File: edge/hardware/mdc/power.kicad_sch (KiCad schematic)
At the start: 1 part, among them J2 Screw_Terminal_01x02

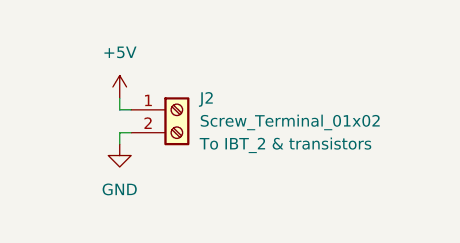
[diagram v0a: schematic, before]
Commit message: rev3.0 schematics
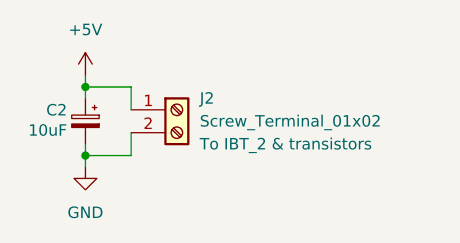
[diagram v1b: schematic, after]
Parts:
- added C2: 10uF, symbol Device:C_Polarized_Small
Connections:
- net +5V: now also C2.1
- net GND: now also C2.2
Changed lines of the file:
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@@
 	(title_block
 		(title "Power")
-		(date "2026-08-08")
+		(date "2026-08-09")
 		(rev "3.0")
 		(comment 1 "Department of EECS- AIoT and Energy Management Lab")
@@
 		(comment 4 "Student: Purit Hongjirakul 黃子奇")
 	)
-	(wire
-		(pts
-			(xy 135.89 100.33) (xy 135.89 99.06)
-		)
-		(stroke
-			(width 0)
-			(type default)
-		)
-	)
-	(wire
-		(pts
-			(xy 135.89 102.87) (xy 137.16 102.87)
-		)
-		(stroke
-			(width 0)
-			(type default)
-		)
-	)
-	(wire
-		(pts
-			(xy 135.89 104.14) (xy 135.89 102.87)
-		)
-		(stroke
-			(width 0)
-			(type default)
-		)
-	)
-	(wire
-		(pts
-			(xy 137.16 100.33) (xy 135.89 100.33)
+	(junction
+		(at 132.08 97.79)
+		(diameter 0)
+		(color 0 0 0 0)
+	)
+	(junction
+		(at 132.08 105.41)
+		(diameter 0)
+		(color 0 0 0 0)
+	)
+	(wire
+		(pts
+			(xy 132.08 106.68) (xy 132.08 105.41)
+		)
+		(stroke
+			(width 0)
+			(type default)
+		)
+	)
+	(wire
+		(pts
+			(xy 132.08 105.41) (xy 132.08 104.14)
+		)
+		(stroke
+			(width 0)
+			(type default)
+		)
+	)
+	(wire
+		(pts
+			(xy 132.08 97.79) (xy 132.08 99.06)
+		)
+		(stroke
+			(width 0)
+			(type default)
+		)
+	)
+	(wire
+		(pts
+			(xy 137.16 105.41) (xy 137.16 102.87)
+		)
+		(stroke
+			(width 0)
+			(type default)
+		)
+	)
+	(wire
+		(pts
+			(xy 132.08 105.41) (xy 137.16 105.41)
+		)
+		(stroke
+			(width 0)
+			(type default)
+		)
+	)
+	(wire
+		(pts
+			(xy 137.16 97.79) (xy 132.08 97.79)
+		)
+		(stroke
+			(width 0)
+			(type default)
+		)
+	)
+	(wire
+		(pts
+			(xy 137.16 97.79) (xy 137.16 100.33)
+		)
+		(stroke
+			(width 0)
+			(type default)
+		)
+	)
+	(wire
+		(pts
+			(xy 132.08 96.52) (xy 132.08 97.79)
 		)
 		(stroke
@@
 	(symbol
 		(lib_id "power:GND")
-		(at 135.89 104.14 0)
+		(at 132.08 106.68 0)
 		(unit 1)
 		(body_style 1)
@@
 		(fields_autoplaced yes)
 		(property "Reference" "#PWR023"
-			(at 135.89 110.49 0)
+			(at 132.08 113.03 0)
 			(hide yes)
 			(show_name no)
@@
 		)
 		(property "Value" "GND"
-			(at 135.89 109.22 0)
+			(at 132.08 111.76 0)
 			(show_name no)
 			(do_not_autoplace no)
@@
 		)
 		(property "Footprint" ""
-			(at 135.89 104.14 0)
+			(at 132.08 106.68 0)
 			(hide yes)
 			(show_name no)
@@
 		)
 		(property "Datasheet" ""
-			(at 135.89 104.14 0)
+			(at 132.08 106.68 0)
 			(hide yes)
 			(show_name no)
@@
 		)
 		(property "Description" "Power symbol creates a global label with name \"GND\" , ground"
-			(at 135.89 104.14 0)
+			(at 132.08 106.68 0)
 			(hide yes)
 			(show_name no)
@@
 	)
 	(symbol
+		(lib_id "Device:C_Polarized_Small")
+		(at 132.08 101.6 0)
+		(mirror y)
+		(unit 1)
+		(body_style 1)
+		(exclude_from_sim no)
+		(in_bom yes)
+		(on_board yes)
+		(in_pos_files yes)
+		(dnp no)
+		(property "Reference" "C2"
+			(at 130.048 100.3682 0)
+			(show_name no)
+			(do_not_autoplace no)
+			(effects
+				(font
+					(size 1.27 1.27)
+				)
+				(justify left)
+			)
+		)
+		(property "Value" "10uF"
+			(at 130.048 102.616 0)
+			(show_name no)
+			(do_not_autoplace no)
+			(effects
+				(font
+					(size 1.27 1.27)
+				)
+				(justify left)
+			)
+		)
+		(property "Footprint" ""
+			(at 132.08 101.6 0)
+			(hide yes)
+			(show_name no)
+			(do_not_autoplace no)
+			(effects
+				(font
+					(size 1.27 1.27)
+				)
+			)
+		)
+		(property "Datasheet" ""
+			(at 132.08 101.6 0)
+			(hide yes)
+			(show_name no)
+			(do_not_autoplace no)
+			(effects
+				(font
+					(size 1.27 1.27)
+				)
+			)
+		)
+		(property "Description" "Polarized capacitor"
+			(at 132.08 101.6 0)
+			(hide yes)
+			(show_name no)
+			(do_not_autoplace no)
+			(effects
+				(font
+					(size 1.27 1.27)
+				)
+			)
+		)
+		(pin "1"
+		)
+		(pin "2"
+		)
+		(instances
+			(project "mdc"
+				(path "/813130ed-0e1e-452d-b14e-fae57783a961/747a2106-db37-4aed-b41f-3c0ea0387f8e"
+					(reference "C2")
+					(unit 1)
+				)
+			)
+		)
+	)
+	(symbol
 		(lib_id "power:+5V")
-		(at 135.89 99.06 0)
+		(at 132.08 96.52 0)
 		(unit 1)
 		(body_style 1)
@@
 		(fields_autoplaced yes)
 		(property "Reference" "#PWR022"
-			(at 135.89 102.87 0)
+			(at 132.08 100.33 0)
 			(hide yes)
 			(show_name no)
@@
 		)
 		(property "Value" "+5V"
-			(at 135.89 93.98 0)
+			(at 132.08 91.44 0)
 			(show_name no)
 			(do_not_autoplace no)
@@
 		)
 		(property "Footprint" ""
-			(at 135.89 99.06 0)
+			(at 132.08 96.52 0)
 			(hide yes)
 			(show_name no)
@@
 		)
 		(property "Datasheet" ""
-			(at 135.89 99.06 0)
+			(at 132.08 96.52 0)
 			(hide yes)
 			(show_name no)
@@
 		)
 		(property "Description" "Power symbol creates a global label with name \"+5V\""
-			(at 135.89 99.06 0)
-			(hide yes)
-			(show_name no)
+			(at 132.08 96.52 0)
+			(hide yes)
+			(show_name no)
